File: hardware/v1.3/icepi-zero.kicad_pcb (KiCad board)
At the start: 4 copper layers, 65 x 30 mm, 160 parts, among them J1 Conn_02x20_Counter_Clockwise, J2 HDMI_C_1.3, J3 USB_C_Receptacle_USB2.0_14P, J4 USB_C_Receptacle_USB2.0_14P, J5 USB_C_Receptacle_USB2.0_14P, J6 Micro_SD_Card_Det2, SW1 SW_Push, SW2 SW_Push, U1 ECP5-CABGA256, U10 W9825G6KH, U11 W25Q128JVS, U2 TLV62569DBV, U3 TLV62569DBV, U4 TLV62569DBV, U5 PCA9306DC1, U6 FT231XQ, U7 TPD2EUSB30A, U8 TPD2EUSB30A, U9 TPD2EUSB30A, Y1 SG-8018CG 50.000000MHz

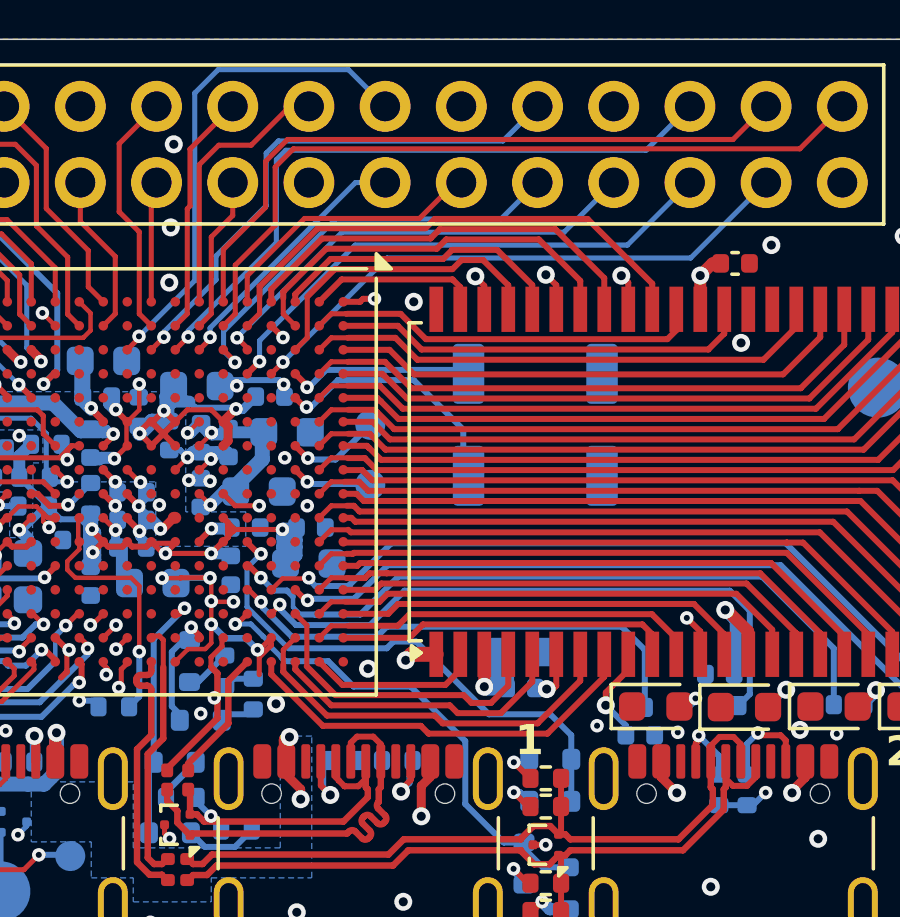
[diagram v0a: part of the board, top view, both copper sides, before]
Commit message: Newest source files
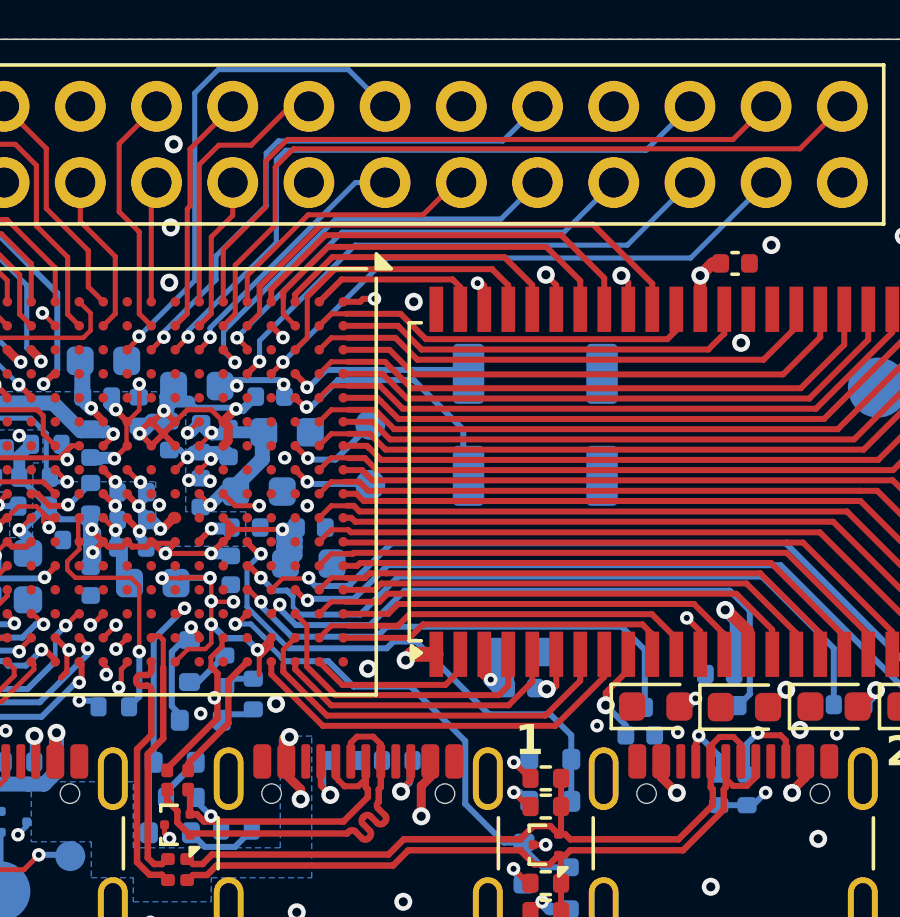
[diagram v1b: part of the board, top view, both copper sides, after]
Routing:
- net +3V3: track 95.9 -> 95.3 mm
